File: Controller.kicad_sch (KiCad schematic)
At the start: 38 parts, among them J1 I2C1, J10 I2C2, J11 MOTOR0_PWR, J12 MOTOR1_PWR, J13 MOTOR2_PWR, J14 MOTOR3_PWR, J15 MOTOR4_PWR, J16 MOTOR5_PWR, J17 ARM0_ROT, J18 ARM0_GRB, J19 ARM1_ROT, J2 I2C1, J20 ARM1_GRB, J21 A0, J22 A1, J23 A2, J24 A3, J25 LED0, J26 LED1, J3 MOTOR0_PWM, J4 MOTOR1_PWM, J5 MOTOR2_PWM, J6 MOTOR3_PWM, J7 MOTOR4_PWM, J8 MOTOR5_PWM, J9 I2C2, Q1 FDB4030L, Q2 FDB4030L, U1 AMS1117-5.0

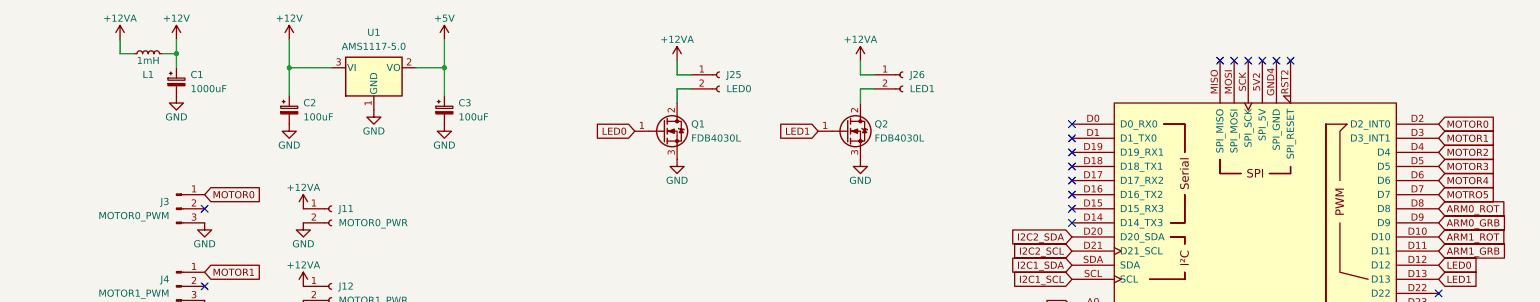
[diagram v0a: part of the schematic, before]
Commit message: Add PCB design, minor corrections on schematic
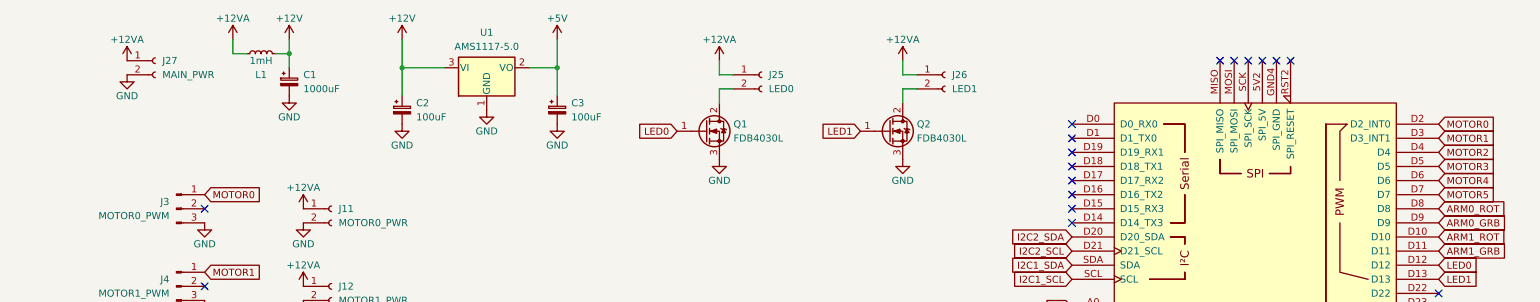
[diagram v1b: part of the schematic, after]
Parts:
- added J27: MAIN_PWR, Controller:ESC-PWR, symbol Connector:Conn_01x02_Female
- J25, J26: footprint Controller:ESC-PWR -> TerminalBlock:TerminalBlock_bornier-2_P5.08mm
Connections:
- net MOTRO5 is gone; now on net MOTOR5: XA1.D7
- net +12VA: now also J27.1 (Pin_1)
- net GND: now also J27.2 (Pin_2)
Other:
- moved on the sheet: C1, C2, C3, J25, J26, L1, Q1, Q2, U1
